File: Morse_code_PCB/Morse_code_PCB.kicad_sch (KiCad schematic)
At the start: 65 parts, among them J1 USB_C_Receptacle_USB2.0, J2 INPUT, J3 OUTPUT, J4 Conn_01x02_Female, J5 Conn_01x04_Female, Q1 AO3400A, Q2 AO3401A, Q3 AO3400A, Q4 AO3401A, SW1 RotaryEncoder_Switch, U1 STM32F030F4Px, U2 OLED_12864, U3 MCP73831-2-OT, U4 CH340E, U5 LP5907MFX-3.3, U6 24AA02-OT, U7 STM32F103C8Tx, Y1 8M, Y2 32.768k

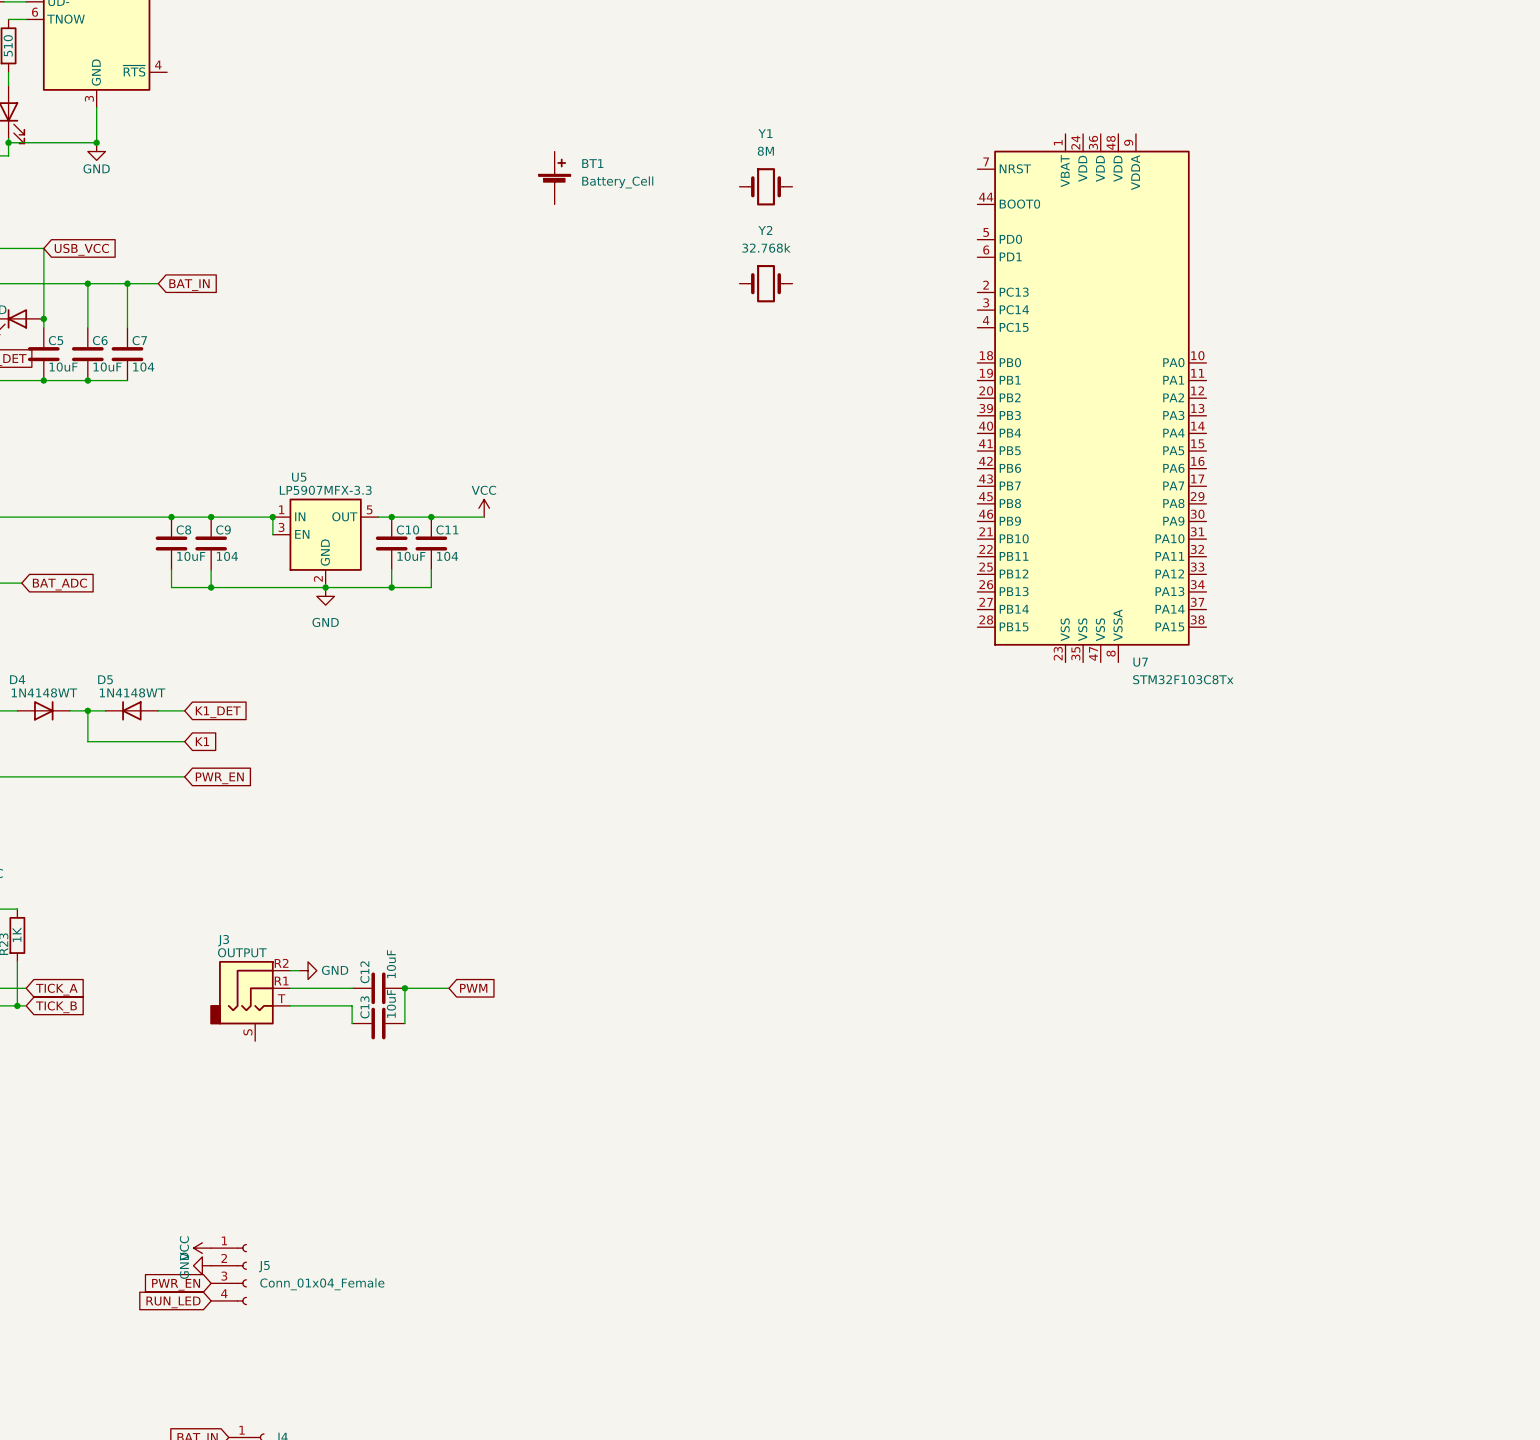
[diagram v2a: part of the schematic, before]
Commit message: updata pcb
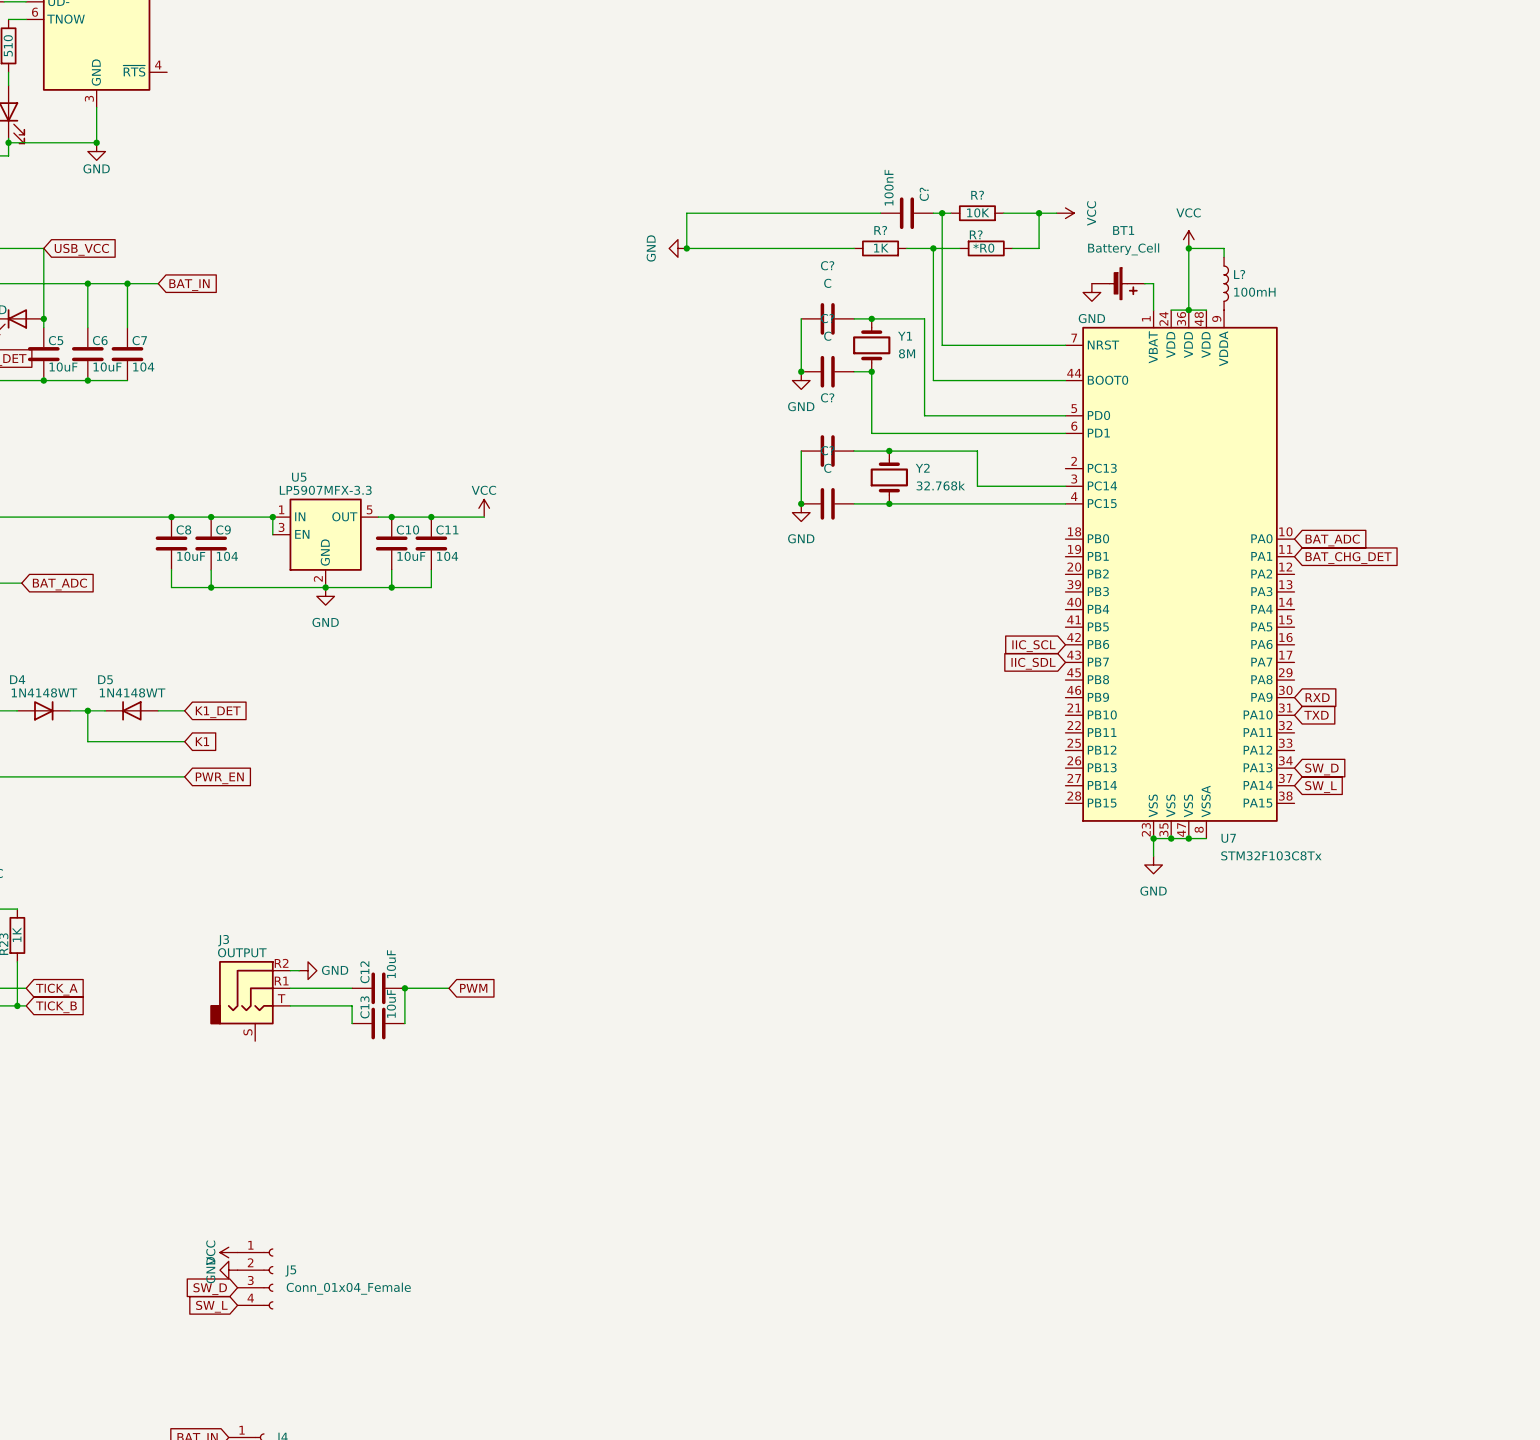
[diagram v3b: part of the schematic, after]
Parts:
- added C? (x3): C, Capacitor_SMD:C_0402_1005Metric_Pad0.74x0.62mm_HandSolder, symbol Device:C
- added C?: 100nF, Capacitor_SMD:C_0805_2012Metric, symbol Device:C
- added C?: (no value), symbol Device:C
- added L?: 100mH, Inductor_SMD:L_0805_2012Metric, symbol Device:L
- added R?: 1K, Resistor_SMD:R_0603_1608Metric, symbol Device:R
- added R?: 10K, Resistor_SMD:R_0603_1608Metric, symbol Device:R
- added R?: *R0, Resistor_SMD:R_0402_1005Metric, symbol Device:R
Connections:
- net BAT_ADC: now also U7.10 (PA0)
- net BAT_CHG_DET: now also U7.11 (PA1)
- net GND: now also BT1.2 (-), U7.23 (VSS), U7.35 (VSS), U7.47 (VSS), U7.8 (VSSA), C?.1, C?.1, C?.1, C?.1, C?.2, R?.1
- net IIC_SCL: now also U7.42 (PB6)
- net IIC_SDL: now also U7.43 (PB7)
- net PWR_EN: no longer J5.3 (Pin_3)
- net RUN_LED: no longer J5.4 (Pin_4)
- net RXD: now also U7.30 (PA9)
- net TXD: now also U7.31 (PA10)
- net VCC: now also U7.24 (VDD), U7.36 (VDD), U7.48 (VDD), L?.1, R?.1, R?.2
- net at U7.1 (VBAT): now also BT1.1 (+)
- net at U7.3 (PC14): now also Y2.2, C?.2
- net SW_D: now reaches U7.34 (PA13)
- net SW_D: now also J5.3 (Pin_3)
- net SW_L: now reaches U7.37 (PA14)
- net SW_L: now also J5.4 (Pin_4)
- net at U7.4 (PC15): now also Y2.1, C?.2
- net at U7.44 (BOOT0): now also R?.2, R?.2
- net at U7.5 (PD0): now also Y1.2, C?.2
- net at U7.6 (PD1): now also Y1.1, C?.2
- net at U7.7 (NRST): now also C?.1, R?.1
- net at U7.9 (VDDA): now also L?.2
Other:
- moved on the sheet: BT1, J5, U7, Y1, Y2

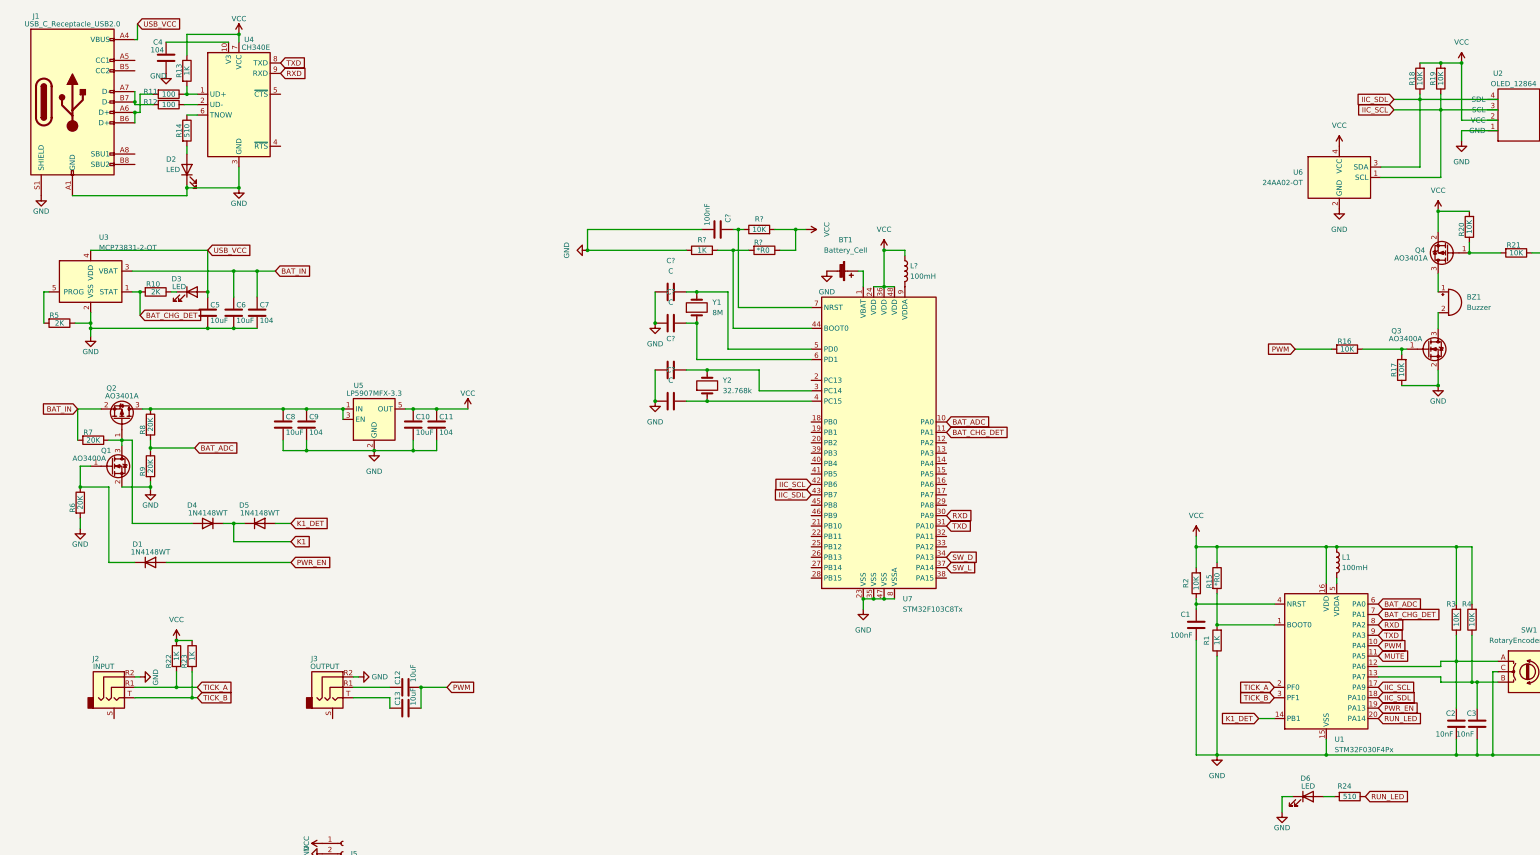
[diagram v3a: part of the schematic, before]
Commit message: Updata PCB Signed-off-by: kevin <kevin@lmve.net>
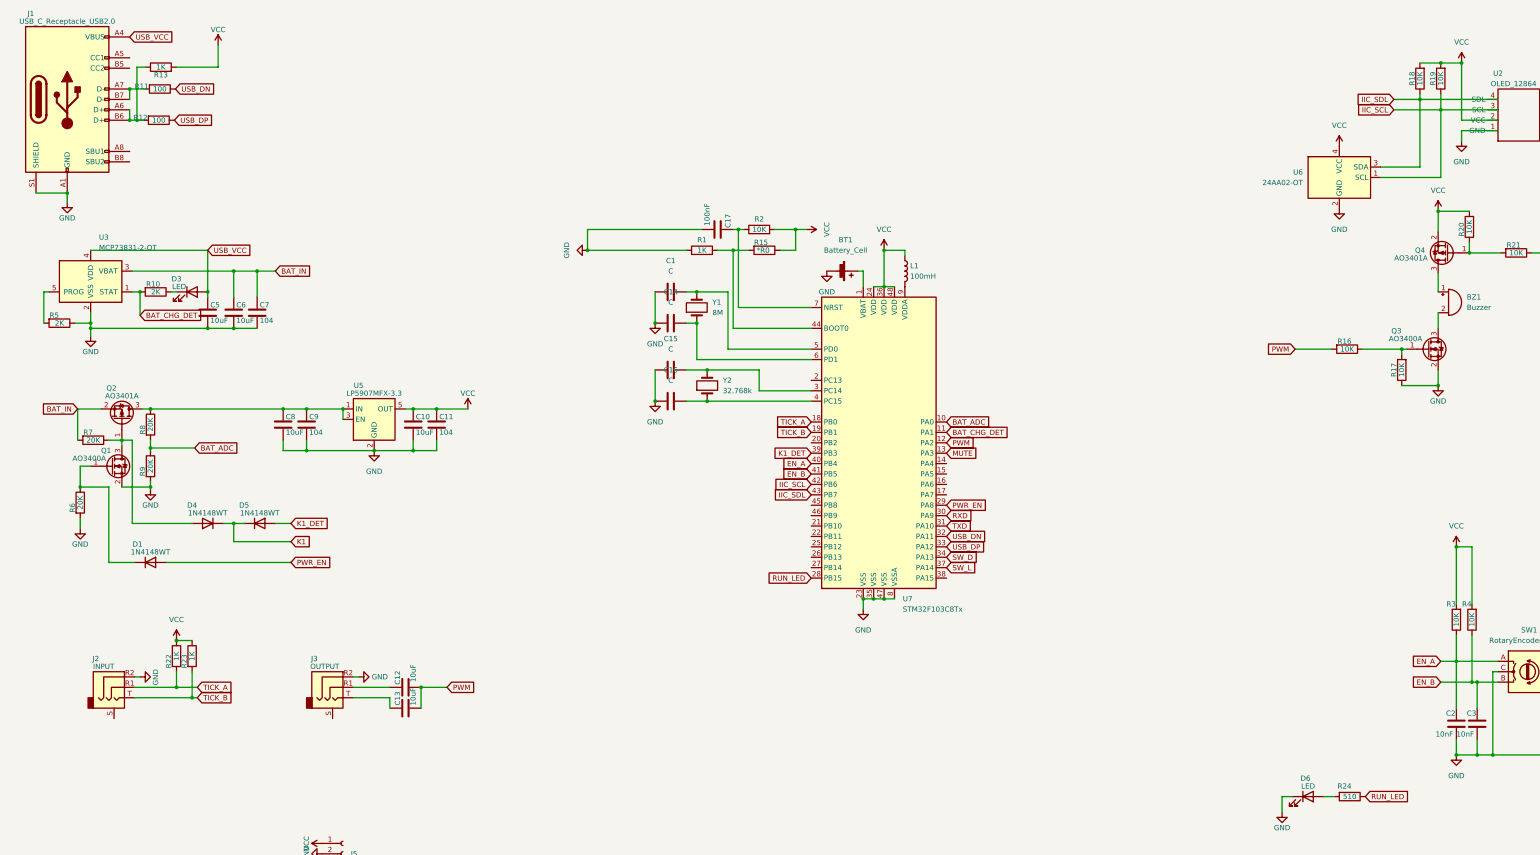
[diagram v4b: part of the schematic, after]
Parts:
- removed C1: 100nF, Capacitor_SMD:C_0805_2012Metric, symbol Device:C
- removed C4: 104, Capacitor_SMD:C_0805_2012Metric, symbol Device:C
- removed D2: LED, LED_SMD:LED_0603_1608Metric, symbol Device:LED
- removed L1: 100mH, Inductor_SMD:L_0805_2012Metric, symbol Device:L
- removed R1: 1K, Resistor_SMD:R_0603_1608Metric, symbol Device:R
- removed R14: 510, Resistor_SMD:R_0603_1608Metric, symbol Device:R
- removed R15: *R0, Resistor_SMD:R_0402_1005Metric, symbol Device:R
- removed R2: 10K, Resistor_SMD:R_0603_1608Metric, symbol Device:R
- removed U1: STM32F030F4Px, Package_SO:TSSOP-20_4.4x6.5mm_P0.65mm, symbol MCU_ST_STM32F0:STM32F030F4Px
- removed U4: CH340E, Package_SO:MSOP-10_3x3mm_P0.5mm, symbol Interface_USB:CH340E
- C15: renamed from C?; value (none) -> C; footprint (none) -> Capacitor_SMD:C_0402_1005Metric_Pad0.74x0.62mm_HandSolder
- gave numbers to parts that had none: 8
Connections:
- net K1_DET: now also U7.39 (PB3)
- net MUTE: now also U7.13 (PA3)
- net PWM: now also U7.12 (PA2)
- net PWR_EN: now also U7.29 (PA8)
- net RUN_LED: now also U7.28 (PB15)
- net TICK_A: now also U7.18 (PB0)
- net TICK_B: now also U7.19 (PB1)
- net VCC: now also R13.2; no longer R13.1
- net USB_DN: now reaches U7.32 (PA11)
- net USB_DN: now also R11.1
- net USB_DP: now reaches U7.33 (PA12)
- net USB_DP: now also R12.1
- net EN_A: now reaches U7.40 (PB4)
- net EN_A: now also C2.1, R3.1, SW1.A
- net EN_B: now reaches U7.41 (PB5)
- net EN_B: now also C3.1, R4.1, SW1.B
- net at J1.A6 (D+), J1.B6 (D+): now also R12.2, R13.1; no longer R11.2
- net at J1.A7 (D-), J1.B7 (D-): now also R11.2; no longer R12.2
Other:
- moved on the sheet: J1, R11, R12, R13
